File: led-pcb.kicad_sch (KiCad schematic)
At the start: 101 parts, among them U1 MAX7221xWG

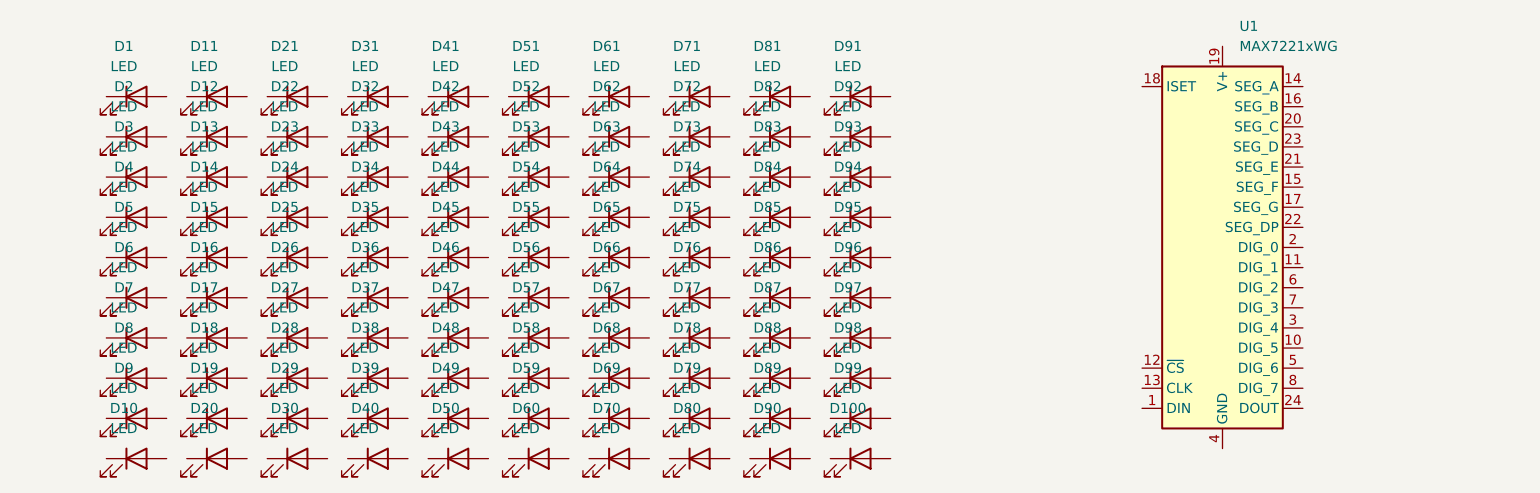
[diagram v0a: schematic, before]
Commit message: e
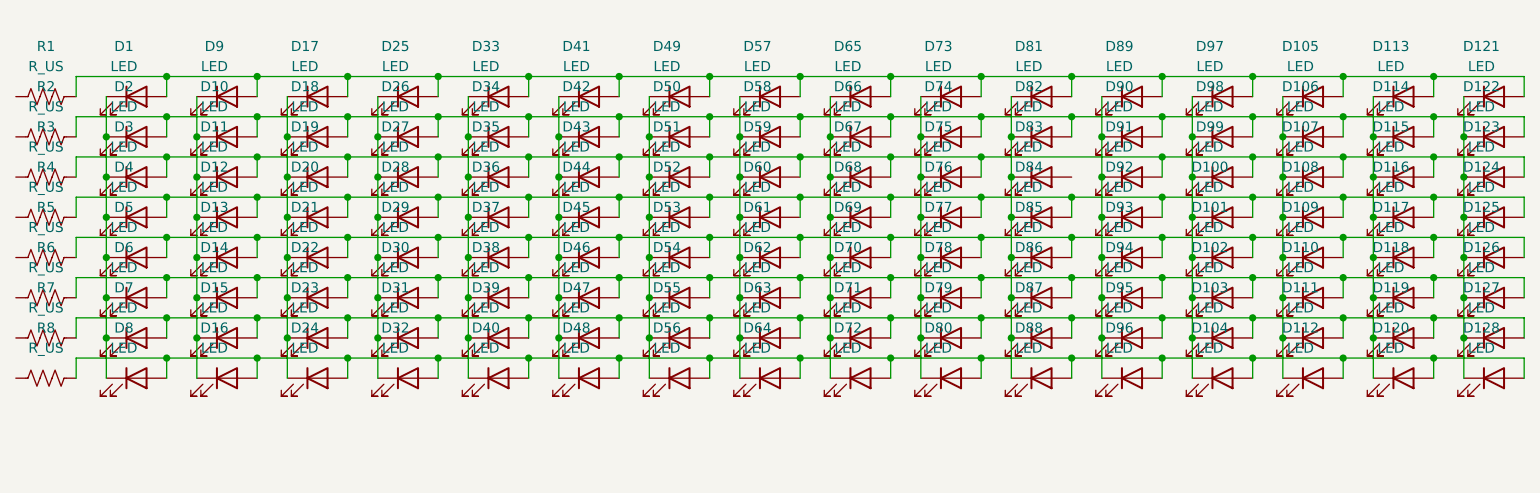
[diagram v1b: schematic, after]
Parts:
- removed U1: MAX7221xWG, Package_SO:SOIC-24W_7.5x15.4mm_P1.27mm, symbol Driver_LED:MAX7221xWG
- added D101, D103, D105, D107, D109, D111, D113, D115, D117, D119, D121, D123, D125, D127: LED, LED_SMD:LED_0603_1608Metric_Pad1.05x0.95mm_HandSolder, symbol Device:LED
- added D102, D104, D106, D108, D110, D112, D114, D116, D118, D120, D122, D124, D126, D128: LED, symbol Device:LED
- added R1, R2, R3, R4, R5, R6, R7, R8: R_US, Resistor_SMD:R_0603_1608Metric, symbol Device:R_US
- D10, D100, D20, D30, D40, D50, D60, D70, D80, D90: footprint LED_SMD:LED_0603_1608Metric_Pad1.05x0.95mm_HandSolder -> (none)
- D19, D29, D39, D49, D59, D69, D79, D89, D9, D99: footprint (none) -> LED_SMD:LED_0603_1608Metric_Pad1.05x0.95mm_HandSolder
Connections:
- net at D49.1 (K): now also D50.1 (K), D51.1 (K), D52.1 (K), D53.1 (K), D54.1 (K), D55.1 (K), D56.1 (K)
- net at D49.2 (A): now also D1.2 (A), D17.2 (A), D25.2 (A), D33.2 (A), D41.2 (A), D57.2 (A), D65.2 (A), D73.2 (A), D81.2 (A), D89.2 (A), D9.2 (A), D97.2 (A), D105.2 (A), D113.2 (A), D121.2 (A), R1.2
- net at D23.1 (K): now also D17.1 (K), D18.1 (K), D19.1 (K), D20.1 (K), D21.1 (K), D22.1 (K), D24.1 (K)
- net at D23.2 (A): now also D15.2 (A), D31.2 (A), D39.2 (A), D47.2 (A), D55.2 (A), D63.2 (A), D7.2 (A), D71.2 (A), D79.2 (A), D87.2 (A), D95.2 (A), D103.2 (A), D111.2 (A), D119.2 (A), D127.2 (A), R7.2
- net at D16.1 (K): now also D10.1 (K), D11.1 (K), D12.1 (K), D13.1 (K), D14.1 (K), D15.1 (K), D9.1 (K)
- net at D16.2 (A): now also D24.2 (A), D32.2 (A), D40.2 (A), D48.2 (A), D56.2 (A), D64.2 (A), D72.2 (A), D8.2 (A), D80.2 (A), D88.2 (A), D96.2 (A), D104.2 (A), D112.2 (A), D120.2 (A), D128.2 (A), R8.2
- net at D100.1 (K): now also D97.1 (K), D98.1 (K), D99.1 (K), D101.1 (K), D102.1 (K), D103.1 (K), D104.1 (K)
- net at D100.2 (A): now also D12.2 (A), D20.2 (A), D28.2 (A), D36.2 (A), D4.2 (A), D44.2 (A), D52.2 (A), D60.2 (A), D68.2 (A), D76.2 (A), D84.2 (A), D92.2 (A), D108.2 (A), D116.2 (A), D124.2 (A), R4.2
- net at D37.1 (K): now also D33.1 (K), D34.1 (K), D35.1 (K), D36.1 (K), D38.1 (K), D39.1 (K), D40.1 (K)
- net at D37.2 (A): now also D13.2 (A), D21.2 (A), D29.2 (A), D45.2 (A), D5.2 (A), D53.2 (A), D61.2 (A), D69.2 (A), D77.2 (A), D85.2 (A), D93.2 (A), D101.2 (A), D109.2 (A), D117.2 (A), D125.2 (A), R5.2
- net at D50.2 (A): now also D10.2 (A), D18.2 (A), D2.2 (A), D26.2 (A), D34.2 (A), D42.2 (A), D58.2 (A), D66.2 (A), D74.2 (A), D82.2 (A), D90.2 (A), D98.2 (A), D106.2 (A), D114.2 (A), D122.2 (A), R2.2
- net at D35.2 (A): now also D11.2 (A), D19.2 (A), D27.2 (A), D3.2 (A), D43.2 (A), D51.2 (A), D59.2 (A), D67.2 (A), D75.2 (A), D91.2 (A), D99.2 (A), D107.2 (A), D115.2 (A), D123.2 (A), R3.2
- net at D43.1 (K): now also D41.1 (K), D42.1 (K), D44.1 (K), D45.1 (K), D46.1 (K), D47.1 (K), D48.1 (K)
- net at D6.1 (K): now also D1.1 (K), D2.1 (K), D3.1 (K), D4.1 (K), D5.1 (K), D7.1 (K), D8.1 (K)
- net at D6.2 (A): now also D14.2 (A), D22.2 (A), D30.2 (A), D38.2 (A), D46.2 (A), D54.2 (A), D62.2 (A), D70.2 (A), D78.2 (A), D86.2 (A), D94.2 (A), D102.2 (A), D110.2 (A), D118.2 (A), D126.2 (A), R6.2
- net at D81.1 (K): now also D82.1 (K), D83.1 (K), D84.1 (K), D85.1 (K), D86.1 (K), D87.1 (K), D88.1 (K)
- net at D63.1 (K): now also D57.1 (K), D58.1 (K), D59.1 (K), D60.1 (K), D61.1 (K), D62.1 (K), D64.1 (K)
- net at D94.1 (K): now also D89.1 (K), D90.1 (K), D91.1 (K), D92.1 (K), D93.1 (K), D95.1 (K), D96.1 (K)
- net at D75.1 (K): now also D73.1 (K), D74.1 (K), D76.1 (K), D77.1 (K), D78.1 (K), D79.1 (K), D80.1 (K)
- net at D25.1 (K): now also D26.1 (K), D27.1 (K), D28.1 (K), D29.1 (K), D30.1 (K), D31.1 (K), D32.1 (K)
- net at D67.1 (K): now also D65.1 (K), D66.1 (K), D68.1 (K), D69.1 (K), D70.1 (K), D71.1 (K), D72.1 (K)
- new net: D113.1 (K), D114.1 (K), D115.1 (K), D116.1 (K), D117.1 (K), D118.1 (K), D119.1 (K), D120.1 (K)
- new net: D121.1 (K), D122.1 (K), D123.1 (K), D124.1 (K), D125.1 (K), D126.1 (K), D127.1 (K), D128.1 (K)
- new net: D105.1 (K), D106.1 (K), D107.1 (K), D108.1 (K), D109.1 (K), D110.1 (K), D111.1 (K), D112.1 (K)
